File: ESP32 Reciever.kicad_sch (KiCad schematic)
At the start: 19 parts, among them J2 Conn_01x10_Pin, J3 Conn_01x10_Pin, J4 TYPE-C-31-M-12, SW1 SW_Push, SW2 SW_Push, U1 LD1117S33TR_SOT223, U2 ESP32-S3-WROOM-1

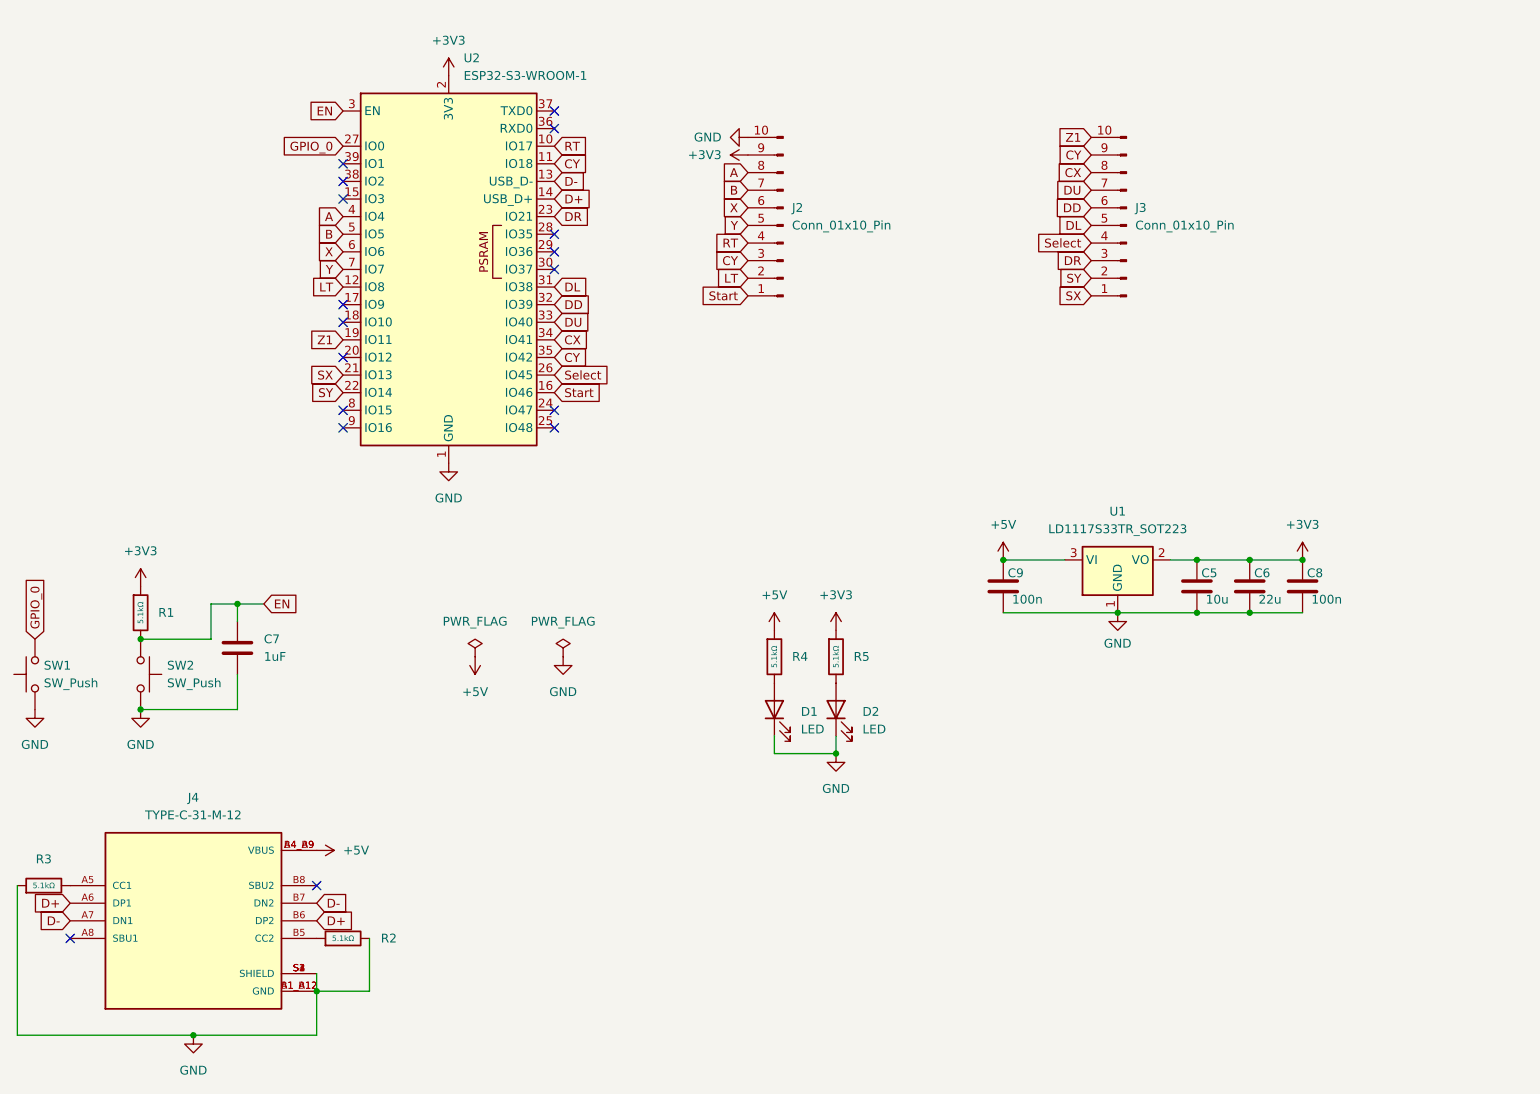
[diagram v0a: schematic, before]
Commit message: Add files via upload
Final PCB and schematic
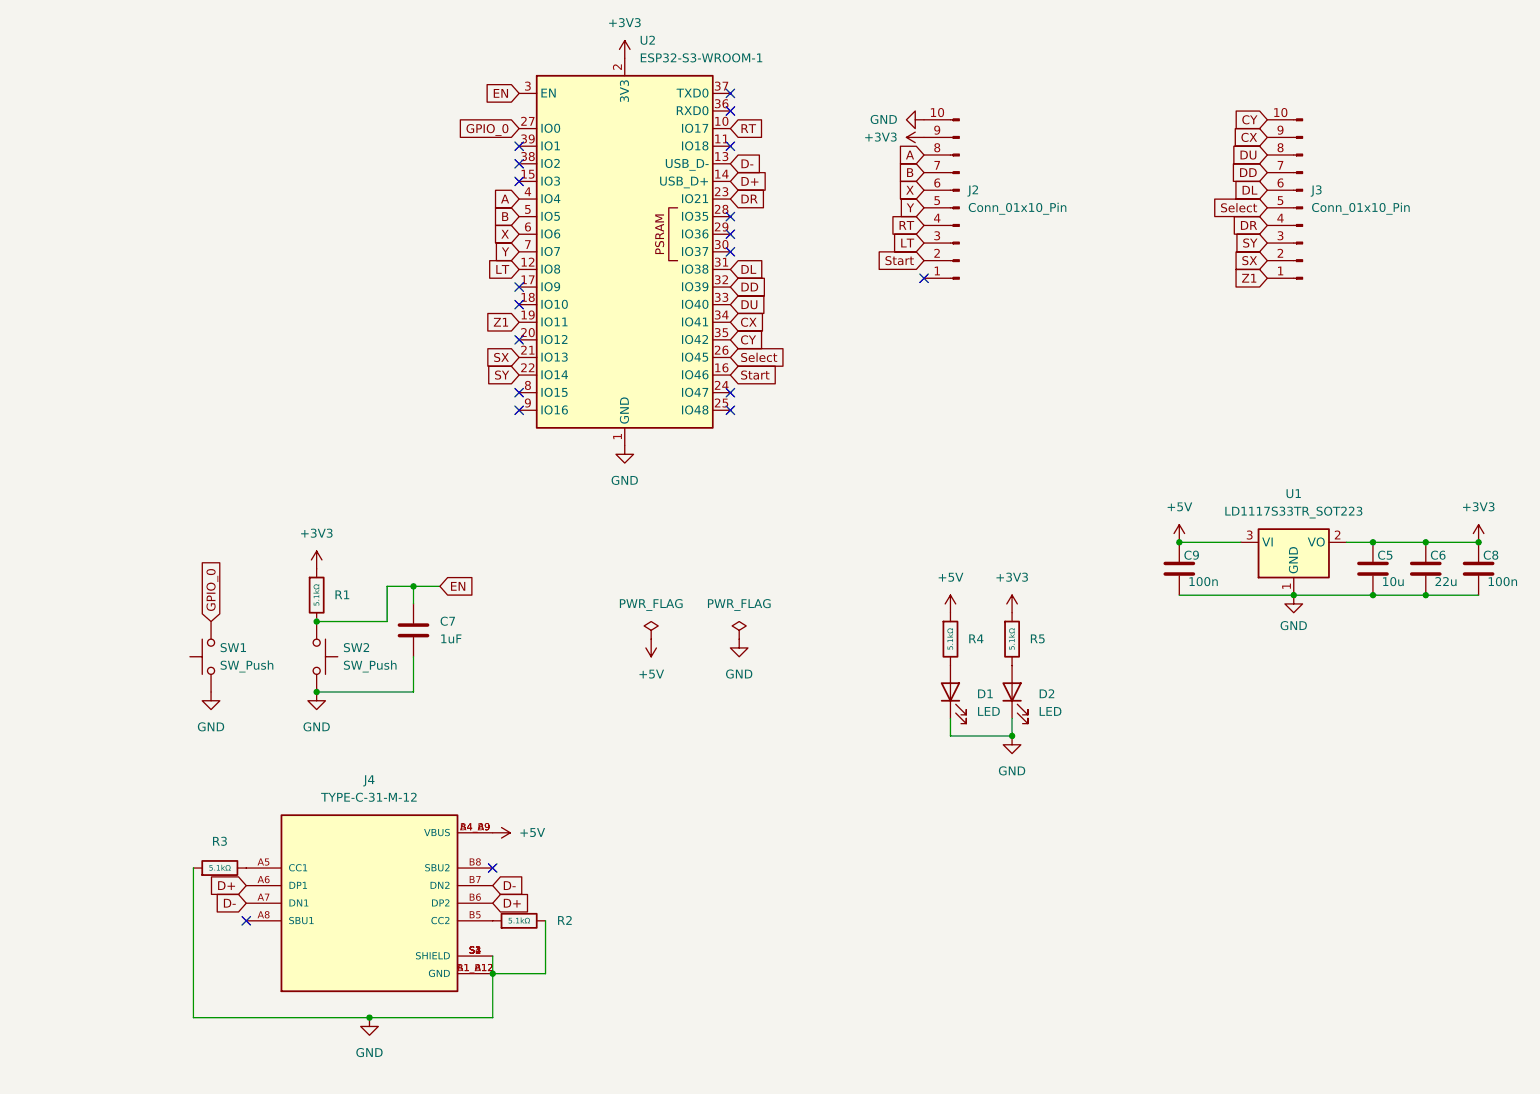
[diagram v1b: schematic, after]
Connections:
- net CX: now also J3.9 (Pin_9); no longer J3.8 (Pin_8)
- net CY: now also J3.10 (Pin_10); no longer J2.3 (Pin_3), J3.9 (Pin_9), U2.11 (IO18)
- net DD: now also J3.7 (Pin_7); no longer J3.6 (Pin_6)
- net DL: now also J3.6 (Pin_6); no longer J3.5 (Pin_5)
- net DR: now also J3.4 (Pin_4); no longer J3.3 (Pin_3)
- net DU: now also J3.8 (Pin_8); no longer J3.7 (Pin_7)
- net LT: now also J2.3 (Pin_3); no longer J2.2 (Pin_2)
- net SX: now also J3.2 (Pin_2); no longer J3.1 (Pin_1)
- net SY: now also J3.3 (Pin_3); no longer J3.2 (Pin_2)
- net Select: now also J3.5 (Pin_5); no longer J3.4 (Pin_4)
- net Start: now also J2.2 (Pin_2); no longer J2.1 (Pin_1)
- net Z1: now also J3.1 (Pin_1); no longer J3.10 (Pin_10)
- no-connect marks 17 -> 19
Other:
- moved on the sheet: C5, C6, C7, C8, C9, D1, D2, J2, J3, J4, R1, R2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
